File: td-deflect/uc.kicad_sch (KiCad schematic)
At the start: 36 parts, among them J15 Conn_01x04_Pin, J16 Conn_02x6_Odd_Even, J2 USB_C_Receptacle_USB2.0, J22 Conn_02x05_Odd_Even, J23 Conn_02x05_Odd_Even, J4 Conn_ARM_JTAG_SWD_10, J6 Conn_01x06_Male, SW1 SW_SPST, U12 AP2204K-3.3, U13 TSOP43xx, U2 STM32G474VETx, U23 AP2204K-5.0, U25 FM24C64B, U4 AP2204K-3.3, U8 INA181, X1 SG-8002CA

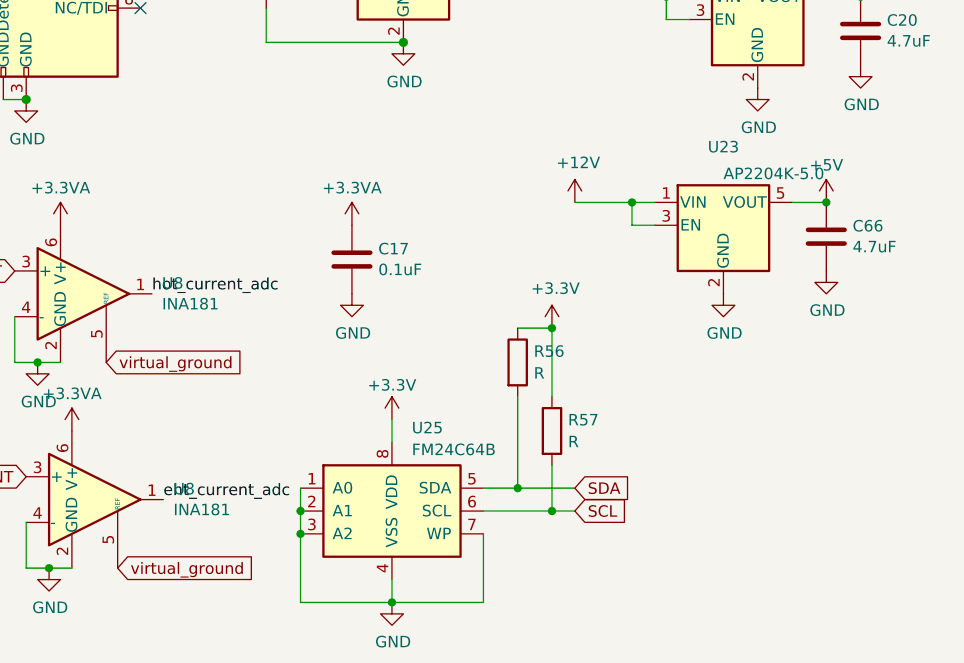
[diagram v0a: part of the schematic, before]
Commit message: update pcb
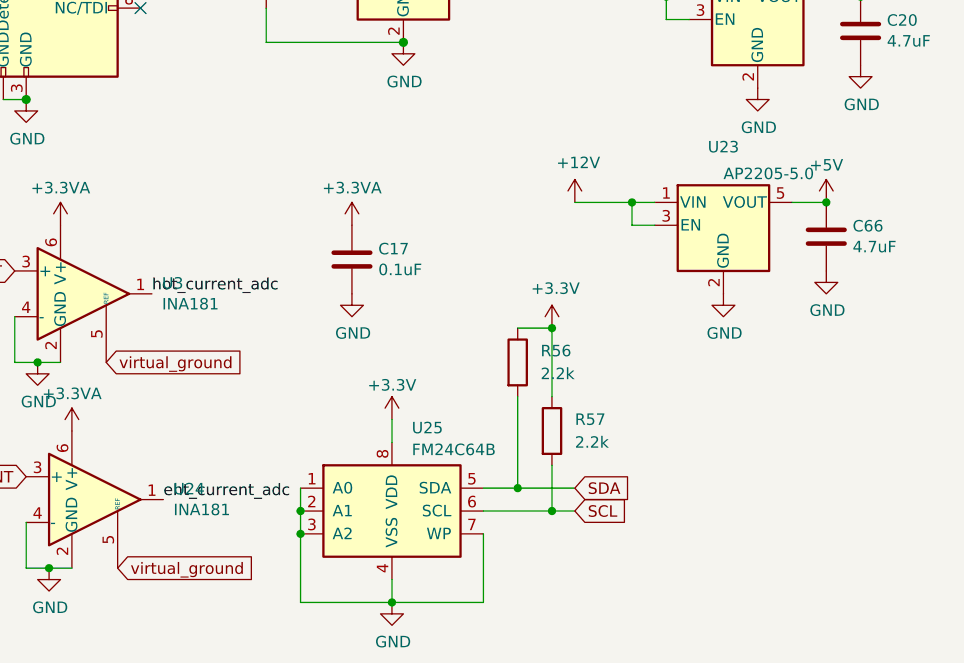
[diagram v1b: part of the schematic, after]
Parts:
- C17, C18, C19, C21, C36, C37, C38, C39, C41: Digikey 1276-1099-1-ND -> 311-1140-1-ND
- F4: Digikey (none) -> 507-1801-1-ND
- J15: Digikey (none) -> 455-B4B-XH-A-ND
- J16: Digikey (none) -> 2057-BHR-12-VUA-ND
- J2: Digikey (none) -> 2073-USB4105-GF-ACT-ND
- J22, J23: Digikey (none) -> 2057-BHR-10-VUA-ND
- J6: Digikey (none) -> DNP
- R112: Digikey (none) -> 311-1.00CRCT-ND
- R12: Digikey (none) -> 311-10.0KCRCT-ND
- R13, R14: Digikey (none) -> 311-5.10KCRCT-ND
- R56, R57: value R -> 2.2k; footprint Resistor_SMD:R_0805_2012Metric_Pad1.20x1.40mm_HandSolder -> Resistor_SMD:R_0805_2012Metric; Digikey (none) -> 311-2.20KCRCT-ND
- SW1: Digikey (none) -> CKN10723CT-ND
- U13: Digikey (none) -> TSOP4338-ND
- U2: Digikey (none) -> 497-19476-ND
- U23: value AP2204K-5.0 -> AP2205-5.0; Digikey (none) -> 31-AP2205-50W5-7CT-ND
- U25: Digikey (none) -> 448-FM24C64B-GTRCT-ND
- renumbered U8 to U24, U8 to U3
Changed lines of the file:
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@@
       (effects (font (size 1.27 1.27)) hide)
     )
-    (property "Digikey" "1276-1099-1-ND" (at 140.97 25.4 0)
+    (property "Digikey" "311-1140-1-ND" (at 140.97 25.4 0)
       (effects (font (size 1.27 1.27)) hide)
     )
@@
       (effects (font (size 1.27 1.27)) hide)
     )
-    (property "Digikey" "1276-1099-1-ND" (at 151.13 25.4 0)
+    (property "Digikey" "311-1140-1-ND" (at 151.13 25.4 0)
       (effects (font (size 1.27 1.27)) hide)
     )
@@
       (effects (font (size 1.27 1.27)) hide)
     )
-    (property "Digikey" "1276-1099-1-ND" (at 161.29 25.4 0)
+    (property "Digikey" "311-1140-1-ND" (at 161.29 25.4 0)
       (effects (font (size 1.27 1.27)) hide)
     )
@@
       (effects (font (size 1.27 1.27)) hide)
     )
-    (property "Digikey" "1276-1099-1-ND" (at 171.45 25.4 0)
+    (property "Digikey" "311-1140-1-ND" (at 171.45 25.4 0)
       (effects (font (size 1.27 1.27)) hide)
     )
@@
       (effects (font (size 1.27 1.27)) hide)
     )
-    (property "Digikey" "1276-1099-1-ND" (at 209.55 91.44 0)
+    (property "Digikey" "311-1140-1-ND" (at 209.55 91.44 0)
       (effects (font (size 1.27 1.27)) hide)
     )
@@
     )
     (property "Datasheet" "~" (at 179.07 48.895 0)
+      (effects (font (size 1.27 1.27)) hide)
+    )
+    (property "Digikey" "DNP" (at 179.07 48.895 0)
       (effects (font (size 1.27 1.27)) hide)
     )
@@
       (effects (font (size 1.27 1.27)) hide)
     )
+    (property "Digikey" "507-1801-1-ND" (at 82.55 184.785 0)
+      (effects (font (size 1.27 1.27)) hide)
+    )
     (pin "2")
     (pin "1")
@@
       (effects (font (size 1.27 1.27)) hide)
     )
+    (property "Digikey" "311-5.10KCRCT-ND" (at 241.3 31.75 0)
+      (effects (font (size 1.27 1.27)) hide)
+    )
     (pin "1")
     (pin "2")
@@
       (effects (font (size 1.27 1.27)))
     )
-    (property "Value" "AP2204K-5.0" (at 260.35 113.665 0)
+    (property "Value" "AP2205-5.0" (at 260.35 113.665 0)
       (effects (font (size 1.27 1.27)) (justify left))
     )
@@
       (effects (font (size 1.27 1.27)) hide)
     )
-    (property "Digikey" "" (at 260.35 119.38 0)
+    (property "Digikey" "31-AP2205-50W5-7CT-ND" (at 260.35 119.38 0)
       (effects (font (size 1.27 1.27)) hide)
     )
@@
   (symbol (lib_id "Amplifier_Current:INA181") (at 189.23 127 0) (unit 1)
     (in_bom yes) (on_board yes) (dnp no)
-    (property "Reference" "U8" (at 197.9676 125.8316 0)
+    (property "Reference" "U3" (at 197.9676 125.8316 0)
       (effects (font (size 1.27 1.27)) (justify left))
     )
@@
     (instances
       (project "td-deflect"
-        (path "/55a1a5e1-4d11-4c3e-b2b4-b9d50ddc5f9d"
-          (reference "U8") (unit 1)
-        )
         (path "/55a1a5e1-4d11-4c3e-b2b4-b9d50ddc5f9d/00000000-0000-0000-0000-00005c37bef7"
           (reference "U3") (unit 1)
@@
       (effects (font (size 1.27 1.27)) hide)
     )
-    (property "Digikey" "1276-1099-1-ND" (at 182.88 25.4 0)
+    (property "Digikey" "311-1140-1-ND" (at 182.88 25.4 0)
       (effects (font (size 1.27 1.27)) hide)
     )
@@
     )
     (property "Datasheet" "~" (at 67.945 183.515 0)
+      (effects (font (size 1.27 1.27)) hide)
+    )
+    (property "Digikey" "455-B4B-XH-A-ND" (at 67.945 183.515 0)
       (effects (font (size 1.27 1.27)) hide)
     )
@@
     )
     (property "Datasheet" "~" (at 35.56 113.03 0)
+      (effects (font (size 1.27 1.27)) hide)
+    )
+    (property "Digikey" "2057-BHR-12-VUA-ND" (at 35.56 113.03 0)
       (effects (font (size 1.27 1.27)) hide)
     )
@@
       (effects (font (size 1.27 1.27)) hide)
     )
-    (property "Digikey" "1276-1099-1-ND" (at 133.35 34.29 0)
+    (property "Digikey" "311-1140-1-ND" (at 133.35 34.29 0)
       (effects (font (size 1.27 1.27)) hide)
     )
@@
       (effects (font (size 1.27 1.27)) hide)
     )
+    (property "Digikey" "CKN10723CT-ND" (at 269.24 27.94 0)
+      (effects (font (size 1.27 1.27)) hide)
+    )
     (pin "1")
     (pin "2")
@@
     )
     (property "Datasheet" "http://www.cypress.com/file/41651/download" (at 223.52 137.16 0)
+      (effects (font (size 1.27 1.27)) hide)
+    )
+    (property "Digikey" "448-FM24C64B-GTRCT-ND" (at 223.52 151.13 0)
       (effects (font (size 1.27 1.27)) hide)
     )
@@
     )
     (property "Datasheet" "https://www.st.com/resource/en/datasheet/stm32g474ve.pdf" (at 119.38 111.76 0)
+      (effects (font (size 1.27 1.27)) hide)
+    )
+    (property "Digikey" "497-19476-ND" (at 119.38 111.76 0)
       (effects (font (size 1.27 1.27)) hide)
     )
@@
       (effects (font (size 1.27 1.27)) hide)
     )
-    (property "Digikey" "1276-1099-1-ND" (at 219.075 123.19 0)
+    (property "Digikey" "311-1140-1-ND" (at 219.075 123.19 0)
       (effects (font (size 1.27 1.27)) hide)
     )
@@
     )
     (property "Datasheet" "~" (at 34.29 171.45 0)
+      (effects (font (size 1.27 1.27)) hide)
+    )
+    (property "Digikey" "2057-BHR-10-VUA-ND" (at 34.29 171.45 0)
       (effects (font (size 1.27 1.27)) hide)
     )
@@
   (symbol (lib_id "Amplifier_Current:INA181") (at 190.5 149.86 0) (unit 1)
     (in_bom yes) (on_board yes) (dnp no)
-    (property "Reference" "U8" (at 199.2376 148.6916 0)
+    (property "Reference" "U24" (at 199.2376 148.6916 0)
       (effects (font (size 1.27 1.27)) (justify left))
     )
@@
     (instances
       (project "td-deflect"
-        (path "/55a1a5e1-4d11-4c3e-b2b4-b9d50ddc5f9d"
-          (reference "U8") (unit 1)
-        )
         (path "/55a1a5e1-4d11-4c3e-b2b4-b9d50ddc5f9d/00000000-0000-0000-0000-00005c37bef7"
           (reference "U24") (unit 1)
@@
     )
     (property "Datasheet" "https://www.usb.org/sites/default/files/documents/usb_type-c.zip" (at 215.9 35.56 0)
+      (effects (font (size 1.27 1.27)) hide)
+    )
+    (property "Digikey" "2073-USB4105-GF-ACT-ND" (at 212.09 35.56 0)
       (effects (font (size 1.27 1.27)) hide)
     )
@@
       (effects (font (size 1.27 1.27)) hide)
     )
-    (property "Digikey" "1276-1099-1-ND" (at 170.18 163.195 0)
+    (property "Digikey" "311-1140-1-ND" (at 170.18 163.195 0)
       (effects (font (size 1.27 1.27)) hide)
     )
@@
   (symbol (lib_id "Device:R") (at 241.3 142.24 0) (unit 1)
     (in_bom yes) (on_board yes) (dnp no) (fields_autoplaced)
-    (property "Reference" "R57" (at 243.078 141.0279 0)
-      (effects (font (size 1.27 1.27)) (justify left))
-    )
-    (property "Value" "R" (at 243.078 143.4521 0)
-      (effects (font (size 1.27 1.27)) (justify left))
-    )
-    (property "Footprint" "Resistor_SMD:R_0805_2012Metric_Pad1.20x1.40mm_HandSolder" (at 239.522 142.24 90)
+    (property "Reference" "R57" (at 243.84 140.97 0)
+      (effects (font (size 1.27 1.27)) (justify left))
+    )
+    (property "Value" "2.2k" (at 243.84 143.51 0)
+      (effects (font (size 1.27 1.27)) (justify left))
+    )
+    (property "Footprint" "Resistor_SMD:R_0805_2012Metric" (at 239.522 142.24 90)
       (effects (font (size 1.27 1.27)) hide)
     )
@@
       (effects (font (size 1.27 1.27)) hide)
     )
+    (property "Digikey" "311-2.20KCRCT-ND" (at 241.3 142.24 0)
+      (effects (font (size 1.27 1.27)) hide)
+    )
     (pin "1")
     (pin "2")
@@
     )
     (property "Datasheet" "~" (at 34.29 151.13 0)
+      (effects (font (size 1.27 1.27)) hide)
+    )
+    (property "Digikey" "2057-BHR-10-VUA-ND" (at 34.29 151.13 0)
       (effects (font (size 1.27 1.27)) hide)
     )
@@
   (symbol (lib_id "Device:R") (at 237.49 134.62 0) (unit 1)
     (in_bom yes) (on_board yes) (dnp no) (fields_autoplaced)
-    (property "Reference" "R56" (at 239.268 133.4079 0)
-      (effects (font (size 1.27 1.27)) (justify left))
-    )
-    (property "Value" "R" (at 239.268 135.8321 0)
-      (effects (font (size 1.27 1.27)) (justify left))
-    )
-    (property "Footprint" "Resistor_SMD:R_0805_2012Metric_Pad1.20x1.40mm_HandSolder" (at 235.712 134.62 90)
+    (property "Reference" "R56" (at 240.03 133.35 0)
+      (effects (font (size 1.27 1.27)) (justify left))
+    )
+    (property "Value" "2.2k" (at 240.03 135.89 0)
+      (effects (font (size 1.27 1.27)) (justify left))
+    )
+    (property "Footprint" "Resistor_SMD:R_0805_2012Metric" (at 235.712 134.62 90)
       (effects (font (size 1.27 1.27)) hide)
     )
@@
       (effects (font (size 1.27 1.27)) hide)
     )
+    (property "Digikey" "311-2.20KCRCT-ND" (at 237.49 134.62 0)
+      (effects (font (size 1.27 1.27)) hide)
+    )
     (pin "1")
     (pin "2")
@@
       (effects (font (size 1.27 1.27)) hide)
     )
+    (property "Digikey" "311-5.10KCRCT-ND" (at 250.19 31.75 0)
+      (effects (font (size 1.27 1.27)) hide)
+    )
     (pin "1")
     (pin "2")
@@
       (effects (font (size 1.27 1.27)) hide)
     )
+    (property "Digikey" "311-10.0KCRCT-ND" (at 269.24 36.83 0)
+      (effects (font (size 1.27 1.27)) hide)
+    )
     (pin "1")
     (pin "2")
@@
       (effects (font (size 1.27 1.27)) hide)
     )
+    (property "Digikey" "TSOP4338-ND" (at 74.93 120.65 0)
+      (effects (font (size 1.27 1.27)) hide)
+    )
     (pin "2")
     (pin "1")
@@
       (effects (font (size 1.27 1.27)) hide)
     )
-    (property "Digikey" "" (at 90.17 41.91 0)
-      (effects (font (size 1.27 1.27)) hide)
-    )
+    (property "Digikey" "311-1.00CRCT-ND" (at 90.17 41.91 0)
+      (effects (font (size 1.27 1.27)) hide)
+    )
